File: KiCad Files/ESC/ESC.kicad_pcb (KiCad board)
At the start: 2 copper layers, 153.2 x 121.6 mm, 97 parts, among them J1 Conn_01x03, J10 Conn_01x03, J11 Conn_01x04, J2 Conn_01x06_Female, J3 Conn_01x01, J4 Conn_01x01, J5 Conn_01x01, J6 Conn_01x03, J7 Conn_01x02, J8 Conn_01x04, J9 Conn_01x03, Q1 IRF3205, Q2 IRF3205, Q3 IRF3205, Q4 IRF3205, Q5 IRF3205, Q6 IRF3205, U1 LM339, U2 L7809, U3 MCP601-xP, U4 IR2110, U5 IR2110, U6 IR2110

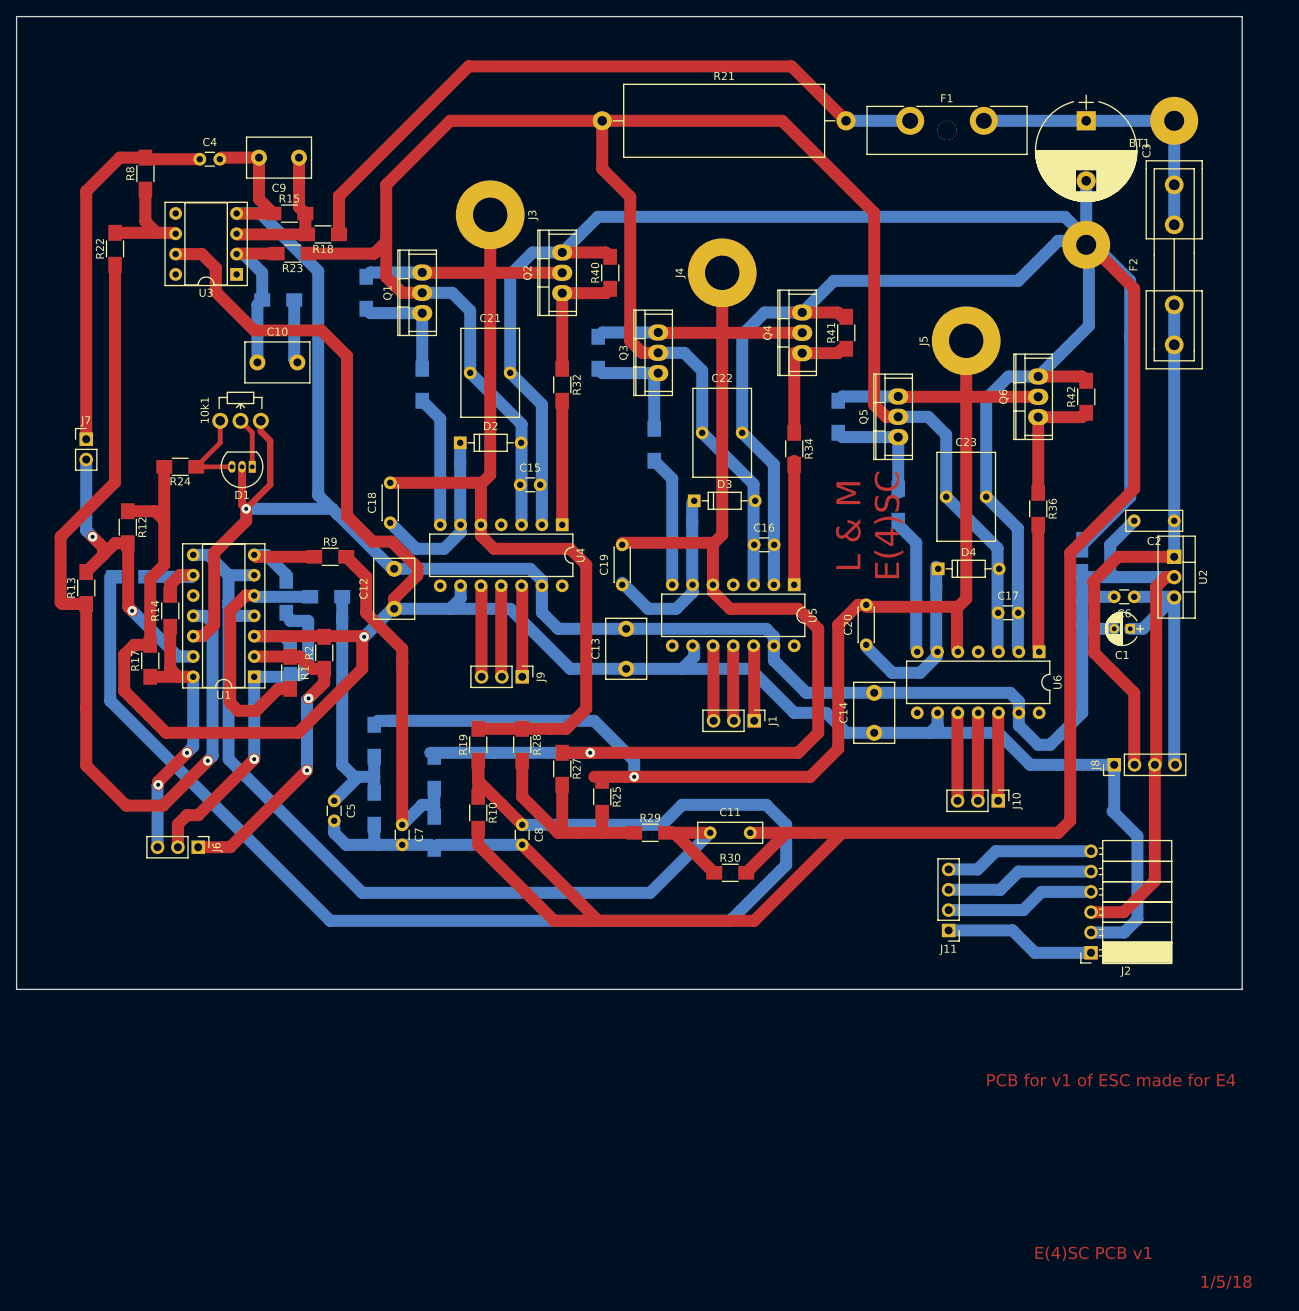
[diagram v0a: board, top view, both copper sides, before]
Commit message: Added PCB v2 and reorganized code
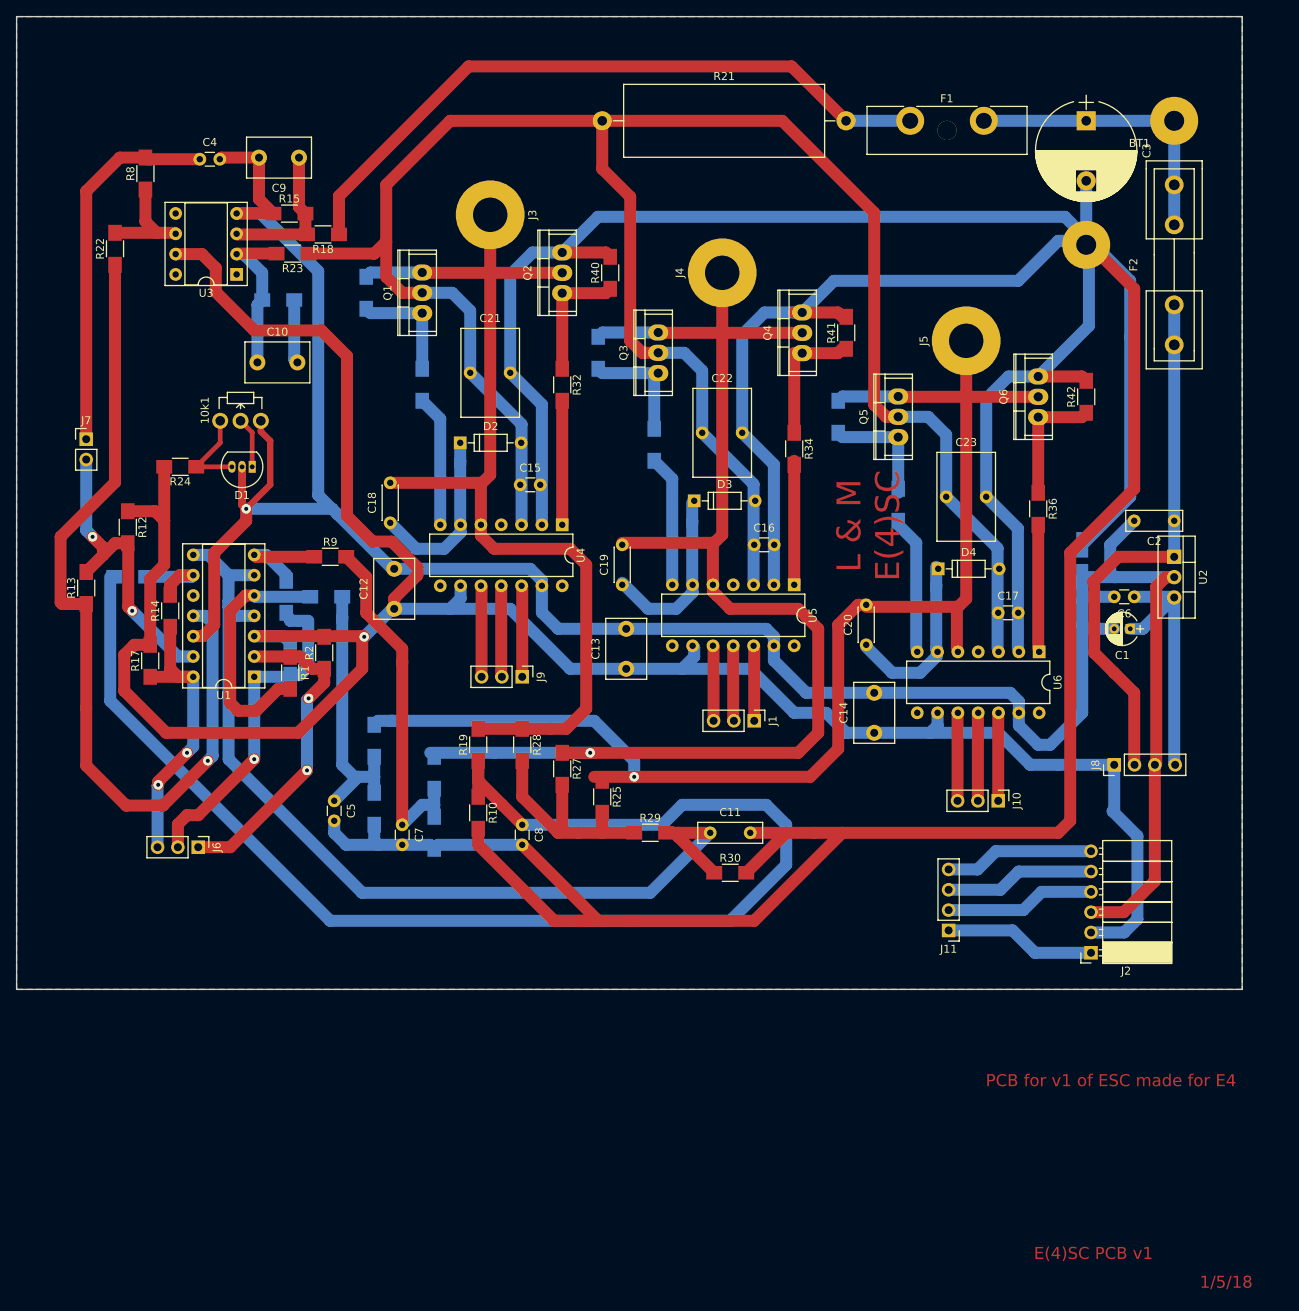
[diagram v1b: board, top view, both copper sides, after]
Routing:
- added copper zone on B.Cu, net LogicGND
- added copper zone on F.Cu, net LogicGND
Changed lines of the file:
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@@
     (links 198)
     (no_connects 18)
-    (area 59.724999 34.924999 213.075001 156.675001)
+    (area 59.724999 34.924999 215.428571 194.55)
     (thickness 1.6)
     (drawings 8)
@@
     (0 F.Cu signal)
     (31 B.Cu signal)
-    (32 B.Adhes user)
-    (33 F.Adhes user)
-    (34 B.Paste user)
-    (35 F.Paste user)
+    (32 B.Adhes user hide)
+    (33 F.Adhes user hide)
+    (34 B.Paste user hide)
+    (35 F.Paste user hide)
     (36 B.SilkS user)
     (37 F.SilkS user)
     (38 B.Mask user)
     (39 F.Mask user)
-    (40 Dwgs.User user)
+    (40 Dwgs.User user hide)
     (41 Cmts.User user)
     (42 Eco1.User user)
@@
     (visible_elements FFFFF77F)
     (pcbplotparams
-      (layerselection 0x00030_80000001)
+      (layerselection 0x000c0_80000001)
       (usegerberextensions false)
       (excludeedgelayer true)
@@
       (plotreference true)
       (plotvalue true)
-      (plotinvisibletext false)
-      (padsonsilk false)
+      (plotinvisibletext true)
+      (padsonsilk true)
       (subtractmaskfromsilk false)
-      (outputformat 1)
+      (outputformat 4)
       (mirror false)
-      (drillshape 1)
+      (drillshape 0)
       (scaleselection 1)
       (outputdirectory ""))
@@
   (segment (start 170.041724 82.527208) (end 170.001724 82.487208) (width 1.5) (layer B.Cu) (net 70))
   (segment (start 177.341724 108.937207) (end 177.341724 114.027208) (width 1.5) (layer F.Cu) (net 70))
+  (zone (net 2) (net_name LogicGND) (layer F.Cu) (hatch edge 0.508)
+    (connect_pads (clearance 0.508))
+    (min_thickness 0.254)
+    (fill yes (arc_segments 16) (thermal_gap 0.508) (thermal_bridge_width 0.508))
+    (polygon
+      (pts
+        (xy 213 156.6) (xy 59.8 156.6) (xy 59.8 35) (xy 213 35)
+      )
+    )
+  )
+  (zone (net 2) (net_name LogicGND) (layer B.Cu) (hatch edge 0.508)
+    (connect_pads (clearance 0.508))
+    (min_thickness 0.254)
+    (fill yes (arc_segments 16) (thermal_gap 0.508) (thermal_bridge_width 0.508))
+    (polygon
+      (pts
+        (xy 213 156.6) (xy 59.8 156.6) (xy 59.8 35) (xy 213 35)
+      )
+    )
+  )
 )
